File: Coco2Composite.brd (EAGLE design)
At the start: 65.1 x 39.7 mm, 20 parts, among them J1 TO_COCO2, J2-SND RCA, J3-COMPOSITE RCA, Q1 BC557, Q2 BC547, U1 MC1372

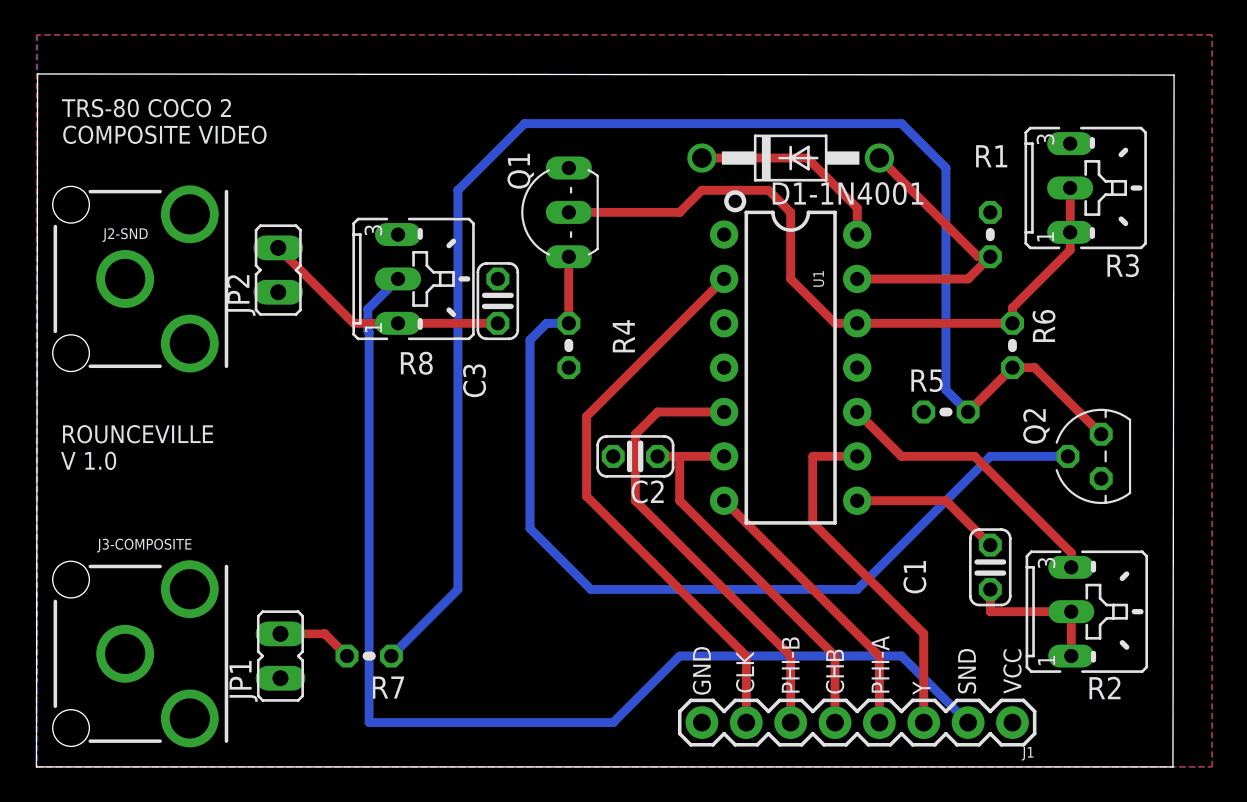
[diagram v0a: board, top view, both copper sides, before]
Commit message: v1.1 revision
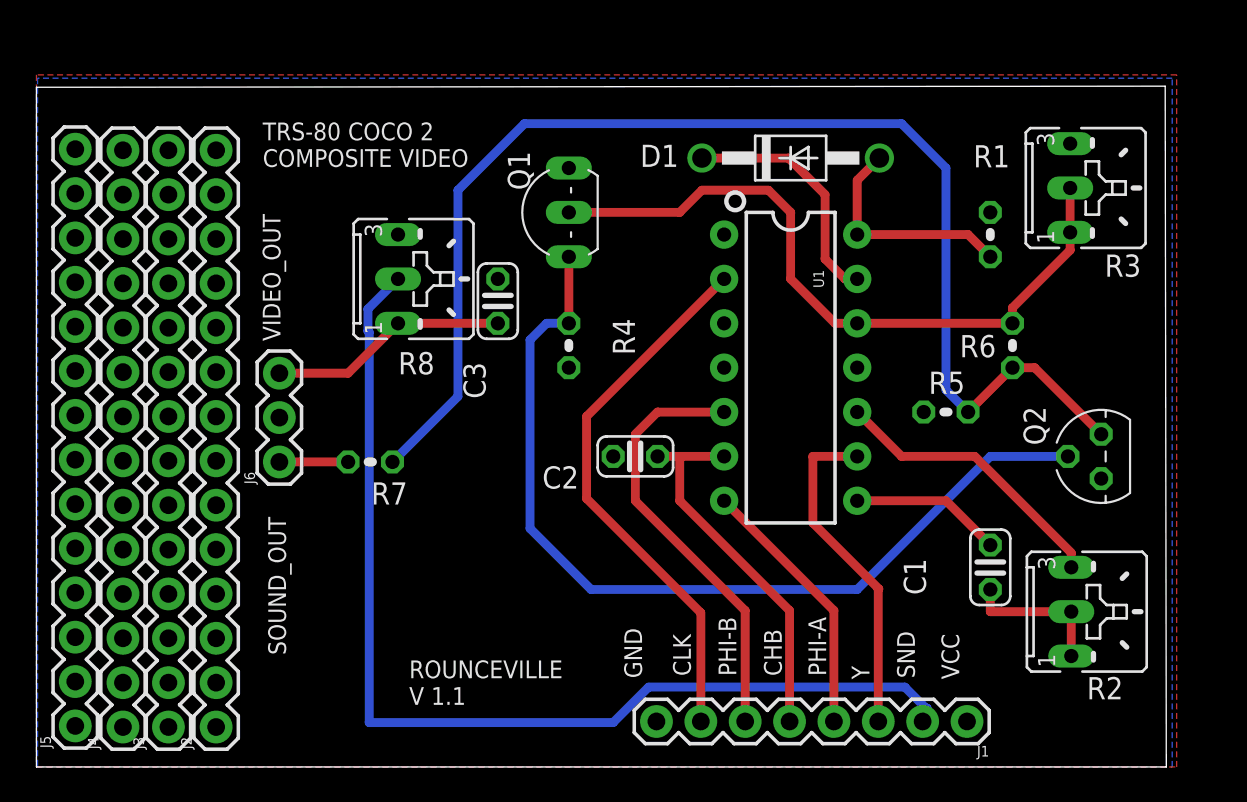
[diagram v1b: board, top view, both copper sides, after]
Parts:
- removed J2-SND, J3-COMPOSITE: RCA, SparkFun-Connectors:RCA
- removed JP1: COMPOSITE_OUT, jumper:JP1
- removed JP2: SOUND_OUT, jumper:JP1
- added J2: JACK_CONN1, SparkFun-Connectors:1X14
- added J3: JACK_CONN2, SparkFun-Connectors:1X14
- added J4: JACK_CONN3, SparkFun-Connectors:1X14
- added J5: JACK_CONN4, SparkFun-Connectors:1X14
- added J6: OUT_JACK, SparkFun-Connectors:1X03
- moved R7 11.1 mm to (19.1, 17.5)
- moved J1 2.60 mm to (53.3, 2.60)
- renumbered D1-1N4001 to D1
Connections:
- net GND: now also J6.2; no longer JP1.1, JP2.1
- net N$1: now also U1.13; no longer U1.14
- net N$10: now also J6.3; no longer JP2.2
- net N$2: now also U1.14; no longer U1.13
- net N$9: now also J6.1; no longer JP1.2
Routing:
- net N$8: track 83.6 -> 72.4 mm
- net N$2: track 16.8 -> 13.1 mm
- net SND: track 63.6 -> 60.3 mm
- net N$1: track 11.6 -> 13.9 mm
- net CLK: track 32.4 -> 31.3 mm
- net PHIB: track 25.8 -> 24.7 mm
- net PHI_A: track 16.4 -> 15.2 mm
- net CHB: track 22.7 -> 21.6 mm
- net Y: track 20.4 -> 19.3 mm
- net N$10: track 14.4 -> 13.7 mm
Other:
- board size 65.1 x 39.7 mm -> 64.7 x 39 mm
- board text added: "ROUNCEVILLE V 1.1"
- board text added: "SOUND_OUT"
- board text added: "VIDEO_OUT"
- board text removed: "ROUNCEVILLE V 1.0"
